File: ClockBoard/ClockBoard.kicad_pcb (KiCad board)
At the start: 2 copper layers, 12 parts, among them J1 Conn_01x04, J2 Conn_01x01, Q1 PN2222A, Q2 PN2222A

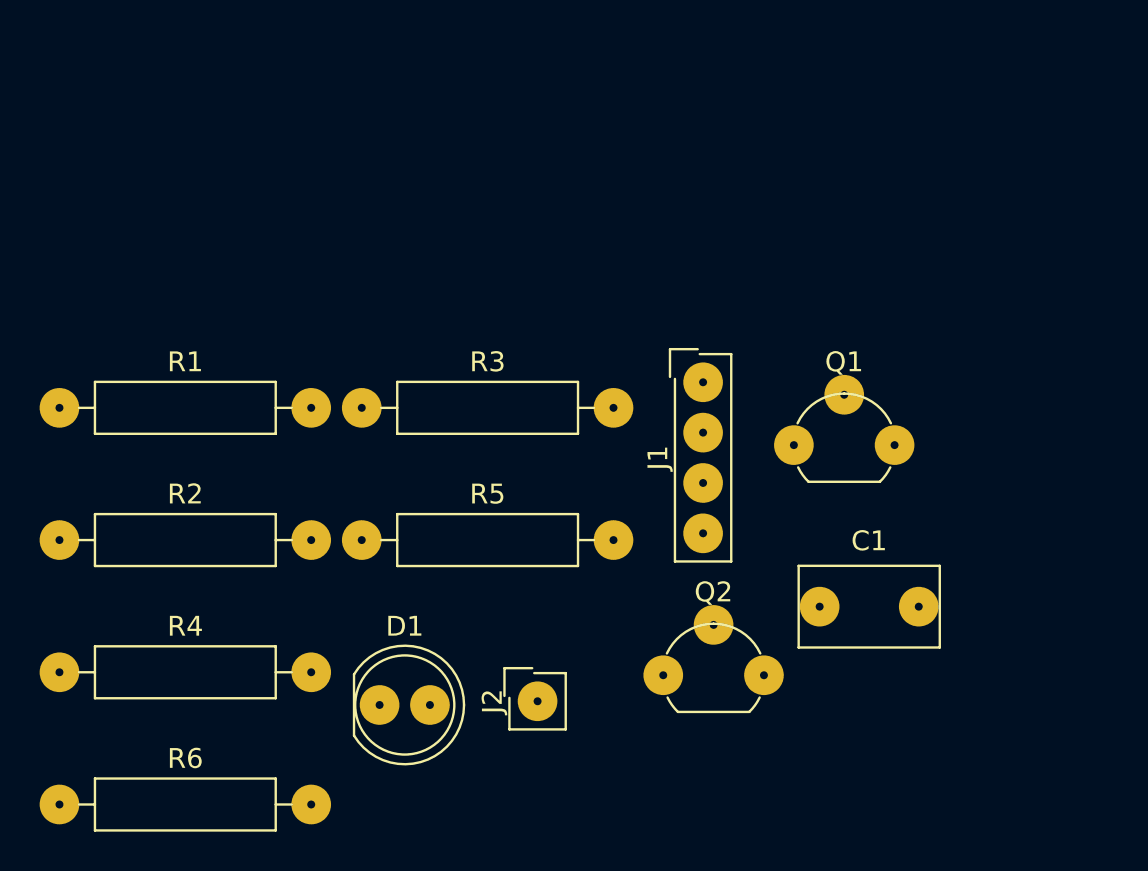
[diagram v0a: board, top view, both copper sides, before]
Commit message: ClockBoard Routed
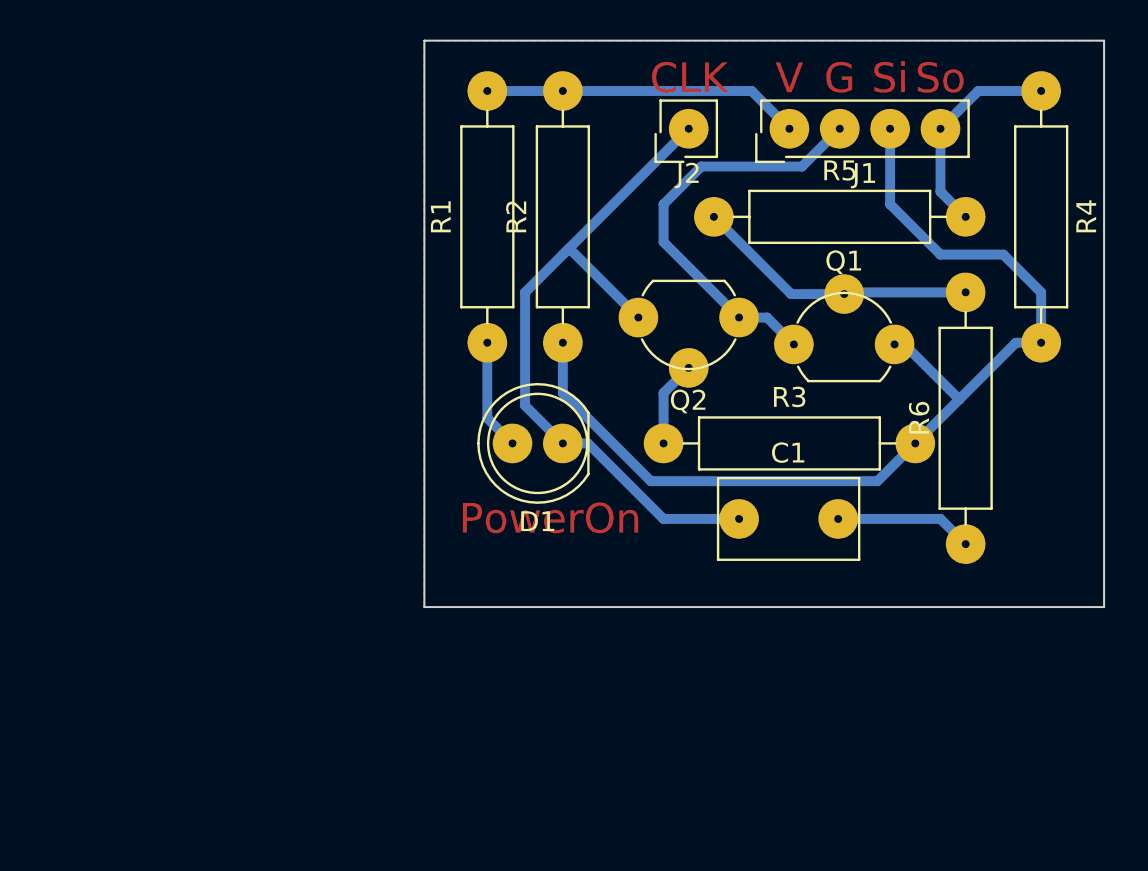
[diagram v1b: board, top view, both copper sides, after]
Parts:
- moved R4 57.6 mm to (189.2, 90.2), turned to 270 degrees
- moved R6 47.6 mm to (185.4, 113.0), turned to 90 degrees
- moved J2 29.9 mm to (171.4, 92.1), turned to 90 degrees
- moved R2 27.3 mm to (165.1, 102.9), turned to 90 degrees
- moved R5 24.1 mm to (172.7, 96.5)
- moved R1 21.8 mm to (161.3, 102.9), turned to 90 degrees
- moved Q2 18.4 mm to (174.0, 101.6), turned to 180 degrees
- moved D1 16.1 mm to (165.1, 108.0), turned to 180 degrees
- moved R3 15.3 mm to (170.2, 108.0)
- moved J1 13.5 mm to (176.5, 92.1), turned to 90 degrees
- moved C1 6.01 mm to (174.0, 111.8)
- moved Q1 5.08 mm to (176.8, 103.0)
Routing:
- net ShortIN: track 0.00 -> 51.6 mm
- net CLK: track 0.00 -> 35.9 mm
- net GND: track 0.00 -> 21.1 mm
- net Vdd: track 0.00 -> 16.0 mm
- net Net-(Q1-Pad2): track 0.00 -> 14.3 mm
- net ShortOUT: track 0.00 -> 10.8 mm
- net Net-(C1-Pad2): track 0.00 -> 6.96 mm
- net Net-(D1-Pad2): track 0.00 -> 5.61 mm
- net Net-(Q2-Pad2): track 0.00 -> 4.34 mm
- added copper zone on B.Cu, net GND
- added copper zone on F.Cu, net GND
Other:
- board outline added: 34.3 x 28.6 mm
- rule via_min_drill: 0.3 -> 0.1
- rule via_min_size: 0.4 -> 0.5
- board text added: "CLK"
- board text added: "G"
- board text added: "PowerOn"
- board text added: "Si"
- board text added: "So"
- board text added: "V"
